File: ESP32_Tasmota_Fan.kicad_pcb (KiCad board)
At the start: 2 copper layers, 70 x 45 mm, 19 parts, among them J1 Conn_01x04, J2 Conn_01x06, J6 Conn_01x02_Female, J8 Conn_01x06, U1 mini_esp32

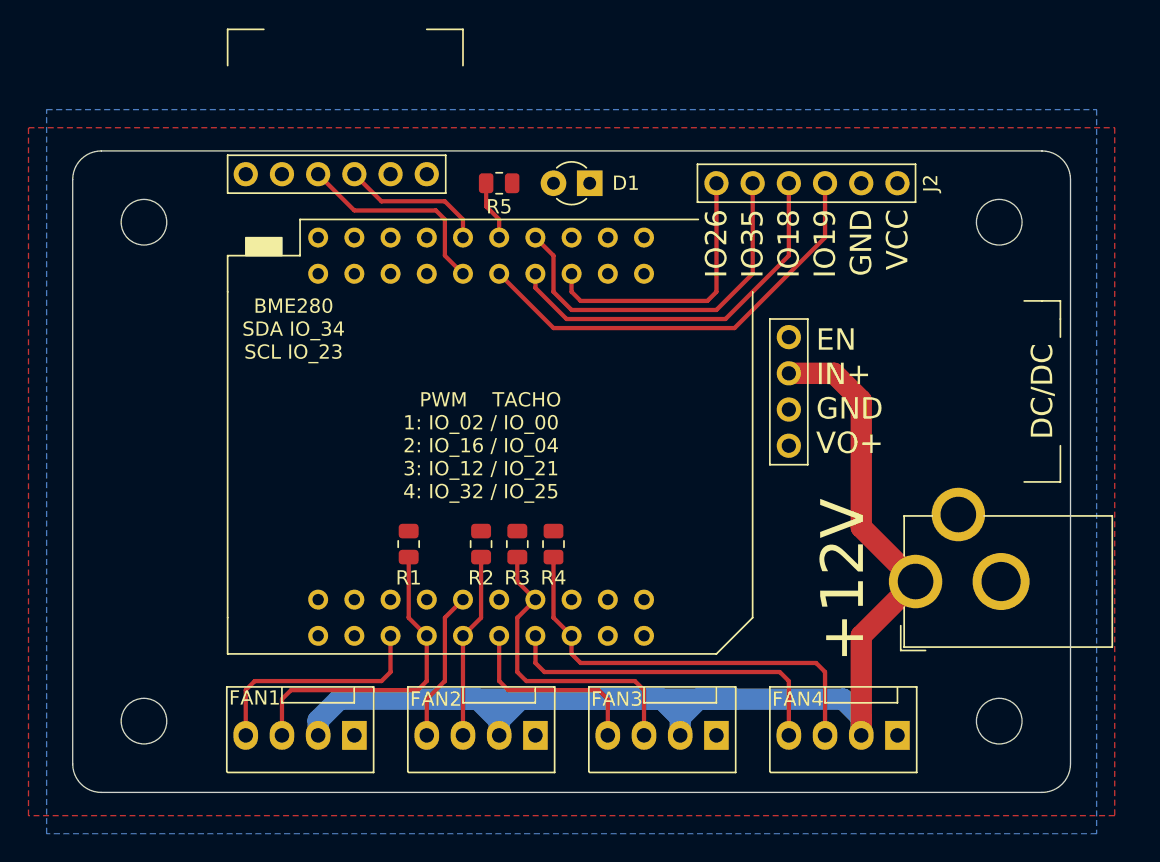
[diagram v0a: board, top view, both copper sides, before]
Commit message: Production Version
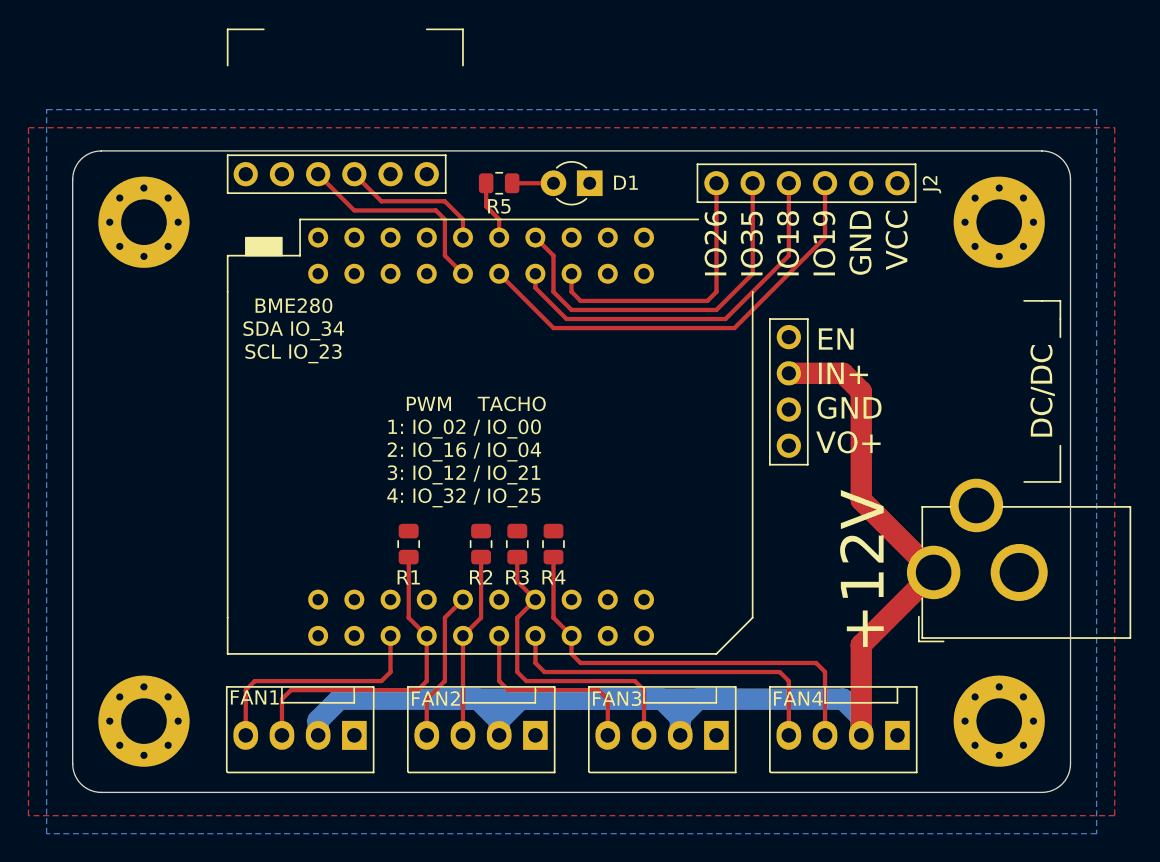
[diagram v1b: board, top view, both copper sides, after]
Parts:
- H1, H2, H3, H4: footprint MountingHole:MountingHole_3.2mm_M3_ISO7380 -> MountingHole:MountingHole_3.2mm_M3_Pad_Via
- moved J6 1.42 mm to (144.8, 133.5)
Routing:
- net Net-(D1-Pad2): track 0.00 -> 2.90 mm
- net +12V: track 99.6 -> 101.1 mm
